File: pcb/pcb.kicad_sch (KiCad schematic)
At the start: 61 parts, among them CN1 Battery, CN10 Pump_On, CN11 Pump_Drain, CN12 Battery_Cell, CN2 Bat_Sense, CN3 VBUS, CN4 3.3V, CN5 VIMM, CN6 ~{Soil_On}, CN7 Soil_Drain, CN8 Soil_Out, CN9 Water_Out, Q2 AO3401A, Q3 AO3400A, Q4 2N7002, U1 USB-C 6PIN, U2 TPS63802DLAT, U3 BQ24075RGTR, U4 TUSB320LIRWBR, U5 ESP-32S DevBoard, U6 Water_Sensor, U7 Pump

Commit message: Renamed the custom library from pcb to custom
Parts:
- U5: footprint pcb:ESP-32S_USB-C_CH340_DevBoard -> custom:ESP-32S_USB-C_CH340_DevBoard; symbol pcb:ESP-32S_USB-C_CH340_DevBoard -> custom:ESP-32S_USB-C_CH340_DevBoard
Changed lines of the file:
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@@
 	)
 	(symbol
-		(lib_id "pcb:ESP-32S_USB-C_CH340_DevBoard")
+		(lib_id "custom:ESP-32S_USB-C_CH340_DevBoard")
 		(at 223.52 72.39 0)
 		(unit 1)
@@
 			)
 		)
-		(property "Footprint" "pcb:ESP-32S_USB-C_CH340_DevBoard"
+		(property "Footprint" "custom:ESP-32S_USB-C_CH340_DevBoard"
 			(at 223.52 54.61 0)
 			(hide yes)

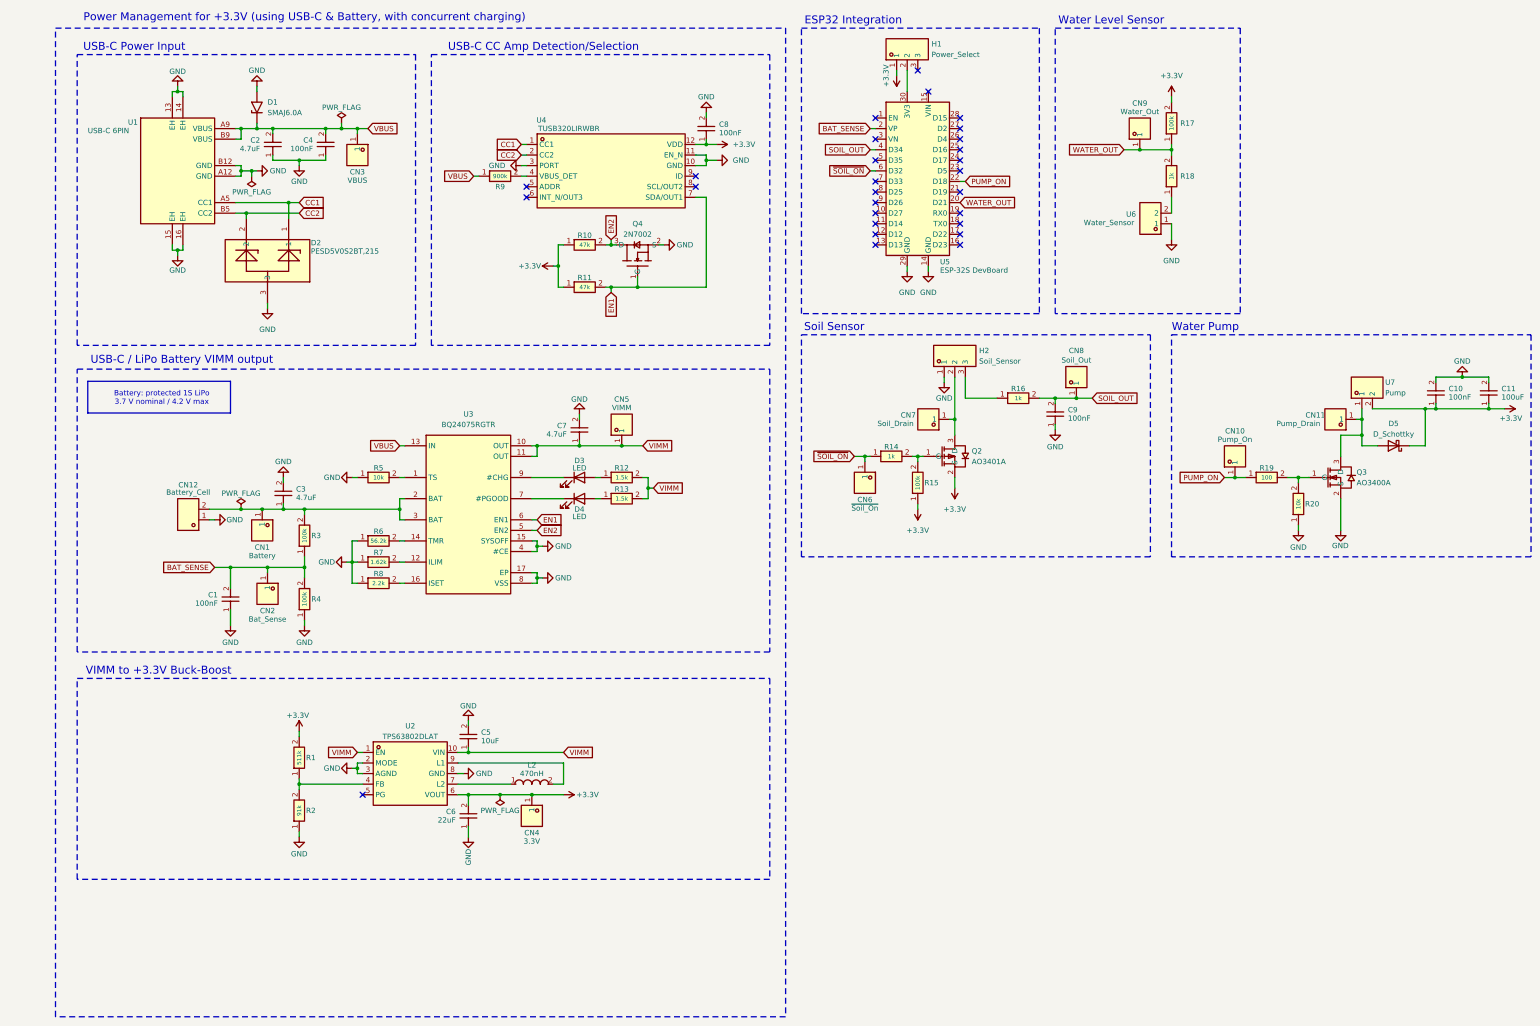
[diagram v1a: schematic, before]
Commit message: Fixed some ERC issues
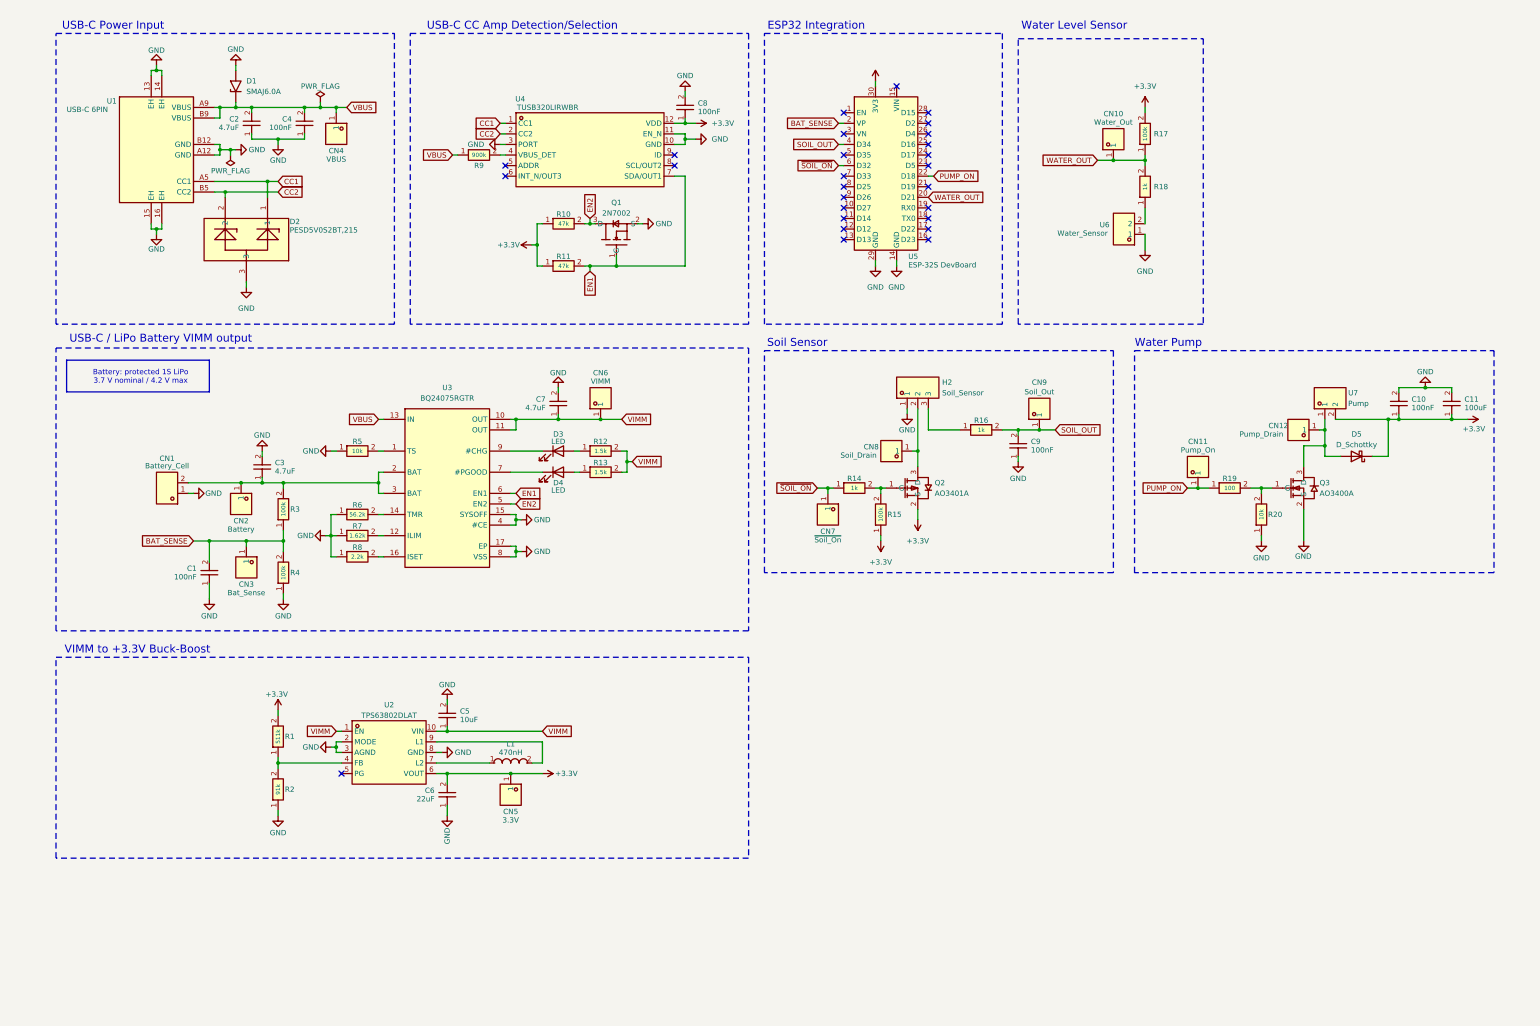
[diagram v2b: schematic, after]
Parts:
- removed H1: Power_Select, EasyEDA:HDR-TH_3P-P2.54-V-M_PZ254V-11-03P, symbol EasyEDA:PZ254V-11-03P_C2937625
- renumbered CN12 to CN1, CN9 to CN10, CN10 to CN11, CN11 to CN12, CN1 to CN2, CN2 to CN3, CN3 to CN4, CN4 to CN5, CN5 to CN6, CN6 to CN7, CN7 to CN8, CN8 to CN9, L2 to L1, Q4 to Q1
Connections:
- net +3.3V: now also U5.30 (3V3)
- no-connect marks 28 -> 27
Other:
- note removed: "Power Management for +3.3V (using USB-C & Battery, with concurrent charging)"
- moved on the sheet: C1, C10, C11, C2, C3, C4, C5, C6, C7, C8, C9, CN1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
